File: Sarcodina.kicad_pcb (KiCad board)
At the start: 2 copper layers, 94 x 94 mm, 375 parts, among them SW1 SW_PUSH, SW10 SW_PUSH, SW11 SW_PUSH, SW12 SW_PUSH, SW13 SW_PUSH, SW14 SW_PUSH, SW15 SW_PUSH, SW16 SW_PUSH, SW17 SW_PUSH, SW18 SW_PUSH, SW19 SW_PUSH, SW2 SW_PUSH, SW20 SW_PUSH, SW21 SW_PUSH, SW22 SW_PUSH, SW23 SW_PUSH, SW24 SW_PUSH, SW25 SW_PUSH, SW3 SW_PUSH, SW4 SW_PUSH, SW5 SW_PUSH, SW6 SW_PUSH, SW7 SW_PUSH, SW8 SW_PUSH, SW9 SW_PUSH

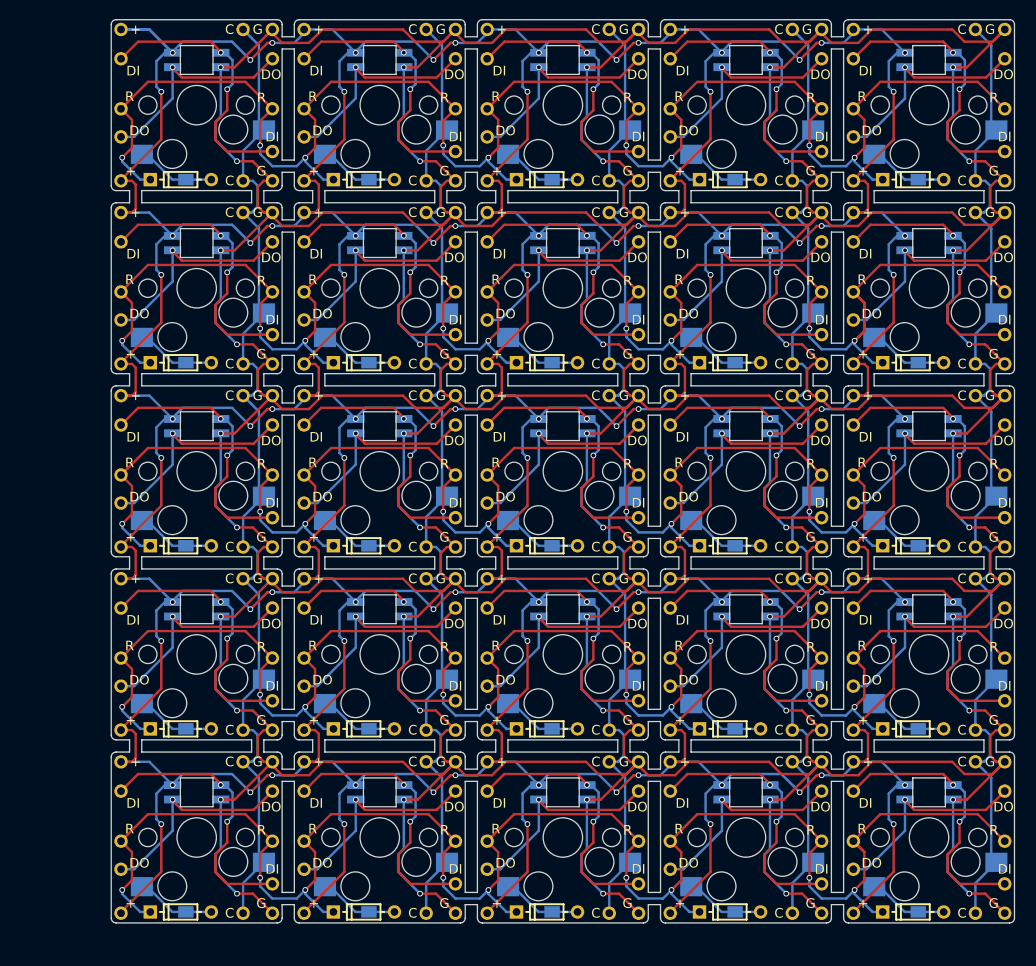
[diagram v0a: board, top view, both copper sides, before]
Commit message: Changed to a develop branch to update the pcb.
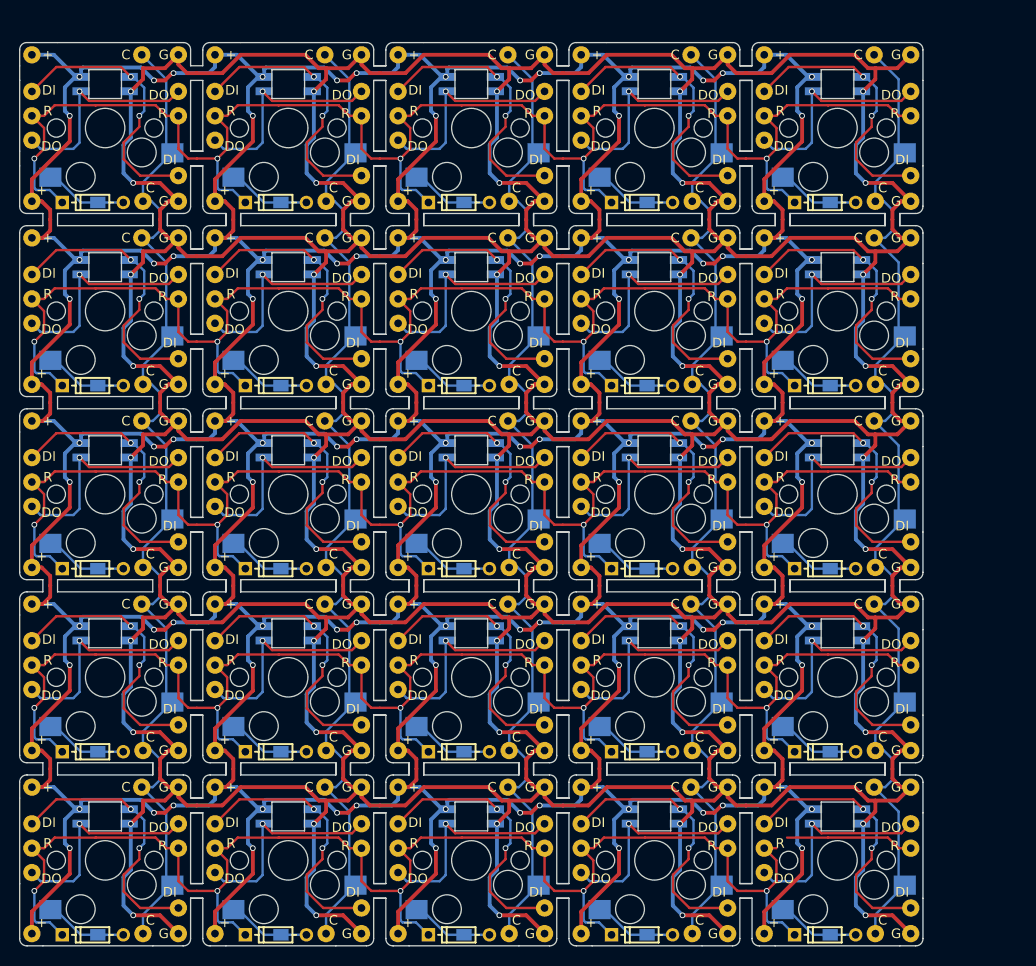
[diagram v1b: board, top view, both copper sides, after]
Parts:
- removed ** (x7), **1, **10, **100, **101, **102, **103, **104, **105, **106, **107, **108, **109, **11, **110, **111, **112, **113, **114, **115, **116, **117, **118, **119, **12, **120, **121, **122, **123, **124, **125, **126, **127, **128, **129, **13, **130, **131, **132, **133, **134, **135, **136, **137, **138, **139, **14, **140, **141, **142, **143, **144, **145, **146, **147, **148, **149, **15, **150, **151, **152, **153, **154, **155, **156, **157, **158, **159, **16, **160, **161, **162, **163, **164, **165, **166, **167, **168, **17, **18, **19, **2, **20, **21, **22, **23, **24, **25, **26, **27, **28, **29, **3, **30, **31, **32, **33, **34, **35, **36, **37, **38, **39, **4, **40, **41, **42, **43, **44, **45, **46, **47, **48, **49, **5, **50, **51, **52, **53, **54, **55, **56, **57, **58, **59, **6, **60, **61, **62, **63, **64, **65, **66, **67, **68, **69, **7, **70, **71, **72, **73, **74, **75, **76, **77, **78, **79, **8, **80, **81, **82, **83, **84, **85, **86, **87, **88, **89, **9, **90, **91, **92, **93, **94, **95, **96, **97, **98, **99: Val**, kbd:1pin_conn_no_silkscreen
- removed 1, 10, 11, 12, 13, 14, 15, 16, 17, 18, 19, 2, 20, 21, 22, 23, 24, 25, 26, 27, 28, 29, 3, 30, 31, 32, 33, 34, 35, 36, 37, 38, 39, 4, 40, 41, 42, 43, 44, 45, 46, 47, 48, 49, 5, 50, 51, 52, 53, 54, 55, 56, 57, 58, 59, 6, 60, 61, 62, 63, 64, 65, 66, 67, 68, 69, 7, 70, 71, 72, 73, 74, 75, 76, 77, 78, 79, 8, 80, 81, 82, 83, 84, 85, 86, 87, 88, 89, 9, 90, 91, 92, 93, 94, 95, 96: , 
- removed the ? at (109.7, 49.3)
- removed the ? at (109.7, 30.2)
- removed the ? at (71.6, 30.2)
- removed the ? at (71.6, 49.3)
- removed the ? at (109.7, 106.4)
- removed the ? at (128.8, 49.3)
- removed the ? at (71.6, 68.3)
- removed the ? at (109.7, 87.4)
- removed the ? at (128.8, 30.2)
- removed the ? at (90.7, 106.4)
- removed the ? at (90.7, 30.2)
- removed the ? at (52.6, 49.3)
- removed the ? at (71.6, 87.4)
- removed the ? at (128.8, 87.4)
- removed the ? at (52.6, 87.4)
- removed the ? at (52.6, 35.4)
- removed the ? at (52.6, 68.3)
- removed the ? at (90.7, 68.3)
- removed the ? at (68.3, 35.4)
- removed the ? at (109.7, 68.3)
- removed the ? at (128.8, 68.3)
- removed the ? at (90.7, 87.4)
- removed the ? at (128.8, 106.4)
- removed the ? at (52.6, 38.4)
- removed the ? at (90.7, 49.3)
- removed the ? at (65.3, 27.2)
- removed the ? at (52.6, 106.4)
- removed the ? at (52.6, 30.2)
- removed the ? at (71.6, 106.4)
- removed the D at (131.8, 119.0)
- removed the D at (55.6, 61.8)
- removed the D at (74.7, 119.0)
- removed the D at (93.7, 80.9)
- removed the D at (112.8, 42.8)
- removed the D at (74.7, 80.9)
- removed the D at (74.7, 99.9)
- removed the D at (93.7, 61.8)
- removed the D at (131.8, 42.8)
- removed the D at (112.8, 99.9)
- removed the D at (112.8, 61.8)
- removed the D at (93.7, 119.0)
- removed the D at (55.6, 80.9)
- removed the D at (55.6, 99.9)
- removed the D at (112.8, 119.0)
- removed the D at (93.7, 42.8)
- removed the D at (74.7, 61.8)
- removed the D at (131.8, 80.9)
- removed the D at (55.6, 119.0)
- removed the D at (74.7, 42.8)
- removed the D at (131.8, 61.8)
- removed the D at (112.8, 80.9)
- removed the D at (55.6, 42.8)
- removed the D at (93.7, 99.9)
- removed the D at (131.8, 99.9)
- removed the L1 at (79.5, 30.4)
- removed the L1 at (136.7, 68.5)
- removed the L1 at (79.5, 87.5)
- removed the L1 at (136.7, 49.4)
- removed the L1 at (79.5, 106.6)
- removed the L1 at (98.6, 87.5)
- removed the L1 at (79.5, 49.4)
- removed the L1 at (60.5, 87.5)
- removed the L1 at (79.5, 68.5)
- removed the L1 at (98.6, 49.4)
- removed the L1 at (136.7, 87.5)
- removed the L1 at (98.6, 106.6)
- removed the L1 at (117.6, 68.5)
- removed the L1 at (98.6, 68.5)
- removed the L1 at (136.7, 106.6)
- removed the L1 at (117.6, 106.6)
- removed the L1 at (136.7, 30.4)
- removed the L1 at (60.5, 30.4)
- removed the L1 at (60.5, 68.5)
- removed the L1 at (117.6, 49.4)
- removed the L1 at (117.6, 30.4)
- removed the L1 at (98.6, 30.4)
- removed the L1 at (60.5, 106.6)
- removed the L1 at (60.5, 49.4)
- removed the L1 at (117.6, 87.5)
- removed SW1, SW10, SW11, SW12, SW13, SW14, SW15, SW16, SW17, SW18, SW19, SW2, SW20, SW21, SW22, SW23, SW24, SW25, SW3, SW4, SW5, SW6, SW8, SW9: SW_PUSH, kbd:CherryMX_Hotswap_single_side
- removed the SW7 at (79.5, 54.1)
- added ?: , , F.Cu at (119.5, 74.3)
- added ?: , , F.Cu at (77.6, 90.8)
- added ?: , , F.Cu at (54.9, 83.2)
- added ?: , , F.Cu at (73.8, 106.0)
- added ?: , , F.Cu at (115.7, 112.4)
- added ?: , , F.Cu at (115.7, 102.2)
- added ?: , , F.Cu at (77.6, 64.1)
- added ?: , , F.Cu at (134.7, 42.4)
- added ?: , , F.Cu at (81.4, 106.0)
- added ?: , , F.Cu at (96.6, 36.2)
- added ?: , , F.Cu at (58.5, 83.2)
- added ?: , , F.Cu at (119.5, 71.7)
- added ?: , , F.Cu at (62.4, 121.3)
- added ?: , , F.Cu at (93.0, 83.2)
- added ?: , , F.Cu at (81.4, 52.7)
- added ?: , , F.Cu at (100.5, 36.2)
- added ?: , , F.Cu at (81.4, 95.9)
- added ?: , , F.Cu at (115.7, 29.8)
- added ?: , , F.Cu at (111.9, 48.9)
- added ?: , , F.Cu at (112.0, 45.1)
- added ?: , , F.Cu at (96.6, 42.4)
- added ?: , , F.Cu at (100.5, 90.8)
- added ?: , , F.Cu at (119.5, 83.2)
- added ?: , , F.Cu at (96.6, 80.5)
- added ?: , , F.Cu at (100.5, 71.7)
- added ?: , , F.Cu at (115.7, 36.2)
- added ?: , , F.Cu at (81.4, 48.9)
- added ?: , , F.Cu at (112.0, 83.2)
- added ?: , , F.Cu at (58.5, 109.8)
- added ?: , , F.Cu at (43.3, 87.0)
- added ?: , , F.Cu at (96.6, 33.6)
- added ?: , , F.Cu at (58.5, 71.7)
- added ?: , , F.Cu at (93.0, 121.3)
- added ?: , , F.Cu at (58.5, 64.1)
- added ?: , , F.Cu at (96.6, 106.0)
- added ?: , , F.Cu at (73.9, 83.2)
- added ?: , , F.Cu at (77.6, 109.8)
- added ?: , , F.Cu at (62.4, 55.2)
- added ?: , , F.Cu at (73.8, 29.8)
- added ?: , , F.Cu at (43.3, 57.8)
- added ?: , , F.Cu at (93.0, 45.1)
- added ?: , , F.Cu at (54.7, 48.9)
- added ?: , , F.Cu at (134.7, 55.2)
- added ?: , , F.Cu at (77.6, 55.2)
- added ?: , , F.Cu at (73.9, 121.3)
- added ?: , , F.Cu at (77.6, 80.5)
- added ?: , , F.Cu at (93.0, 64.1)
- added ?: , , F.Cu at (43.3, 121.3)
- added ?: , , F.Cu at (131.1, 64.1)
- added ?: , , F.Cu at (134.7, 109.8)
- added ?: , , F.Cu at (119.5, 45.1)
- added ?: , , F.Cu at (130.9, 29.8)
- added ?: , , F.Cu at (96.6, 29.8)
- added ?: , , F.Cu at (115.7, 87.0)
- added ?: , , F.Cu at (131.1, 83.2)
- added ?: , , F.Cu at (134.7, 99.5)
- added ?: , , F.Cu at (100.5, 95.9)
- added ?: , , F.Cu at (134.7, 36.2)
- added ?: , , F.Cu at (62.4, 106.0)
- added ?: , , F.Cu at (134.7, 93.3)
- added ?: , , F.Cu at (81.4, 83.2)
- added ?: , , F.Cu at (77.6, 99.5)
- added ?: , , F.Cu at (115.7, 109.8)
- added ?: , , F.Cu at (92.8, 106.0)
- added ?: , , F.Cu at (62.4, 36.2)
- added ?: , , F.Cu at (134.7, 33.6)
- added ?: , , F.Cu at (100.5, 83.2)
- added ?: , , F.Cu at (100.5, 67.9)
- added ?: , , F.Cu at (100.5, 114.9)
- added ?: , , F.Cu at (81.4, 76.8)
- added ?: , , F.Cu at (62.4, 57.8)
- added ?: , , F.Cu at (81.4, 38.7)
- added ?: , , F.Cu at (81.4, 29.8)
- added ?: , , F.Cu at (77.6, 33.6)
- added ?: , , F.Cu at (62.4, 71.7)
- added ?: , , F.Cu at (58.5, 106.0)
- added ?: , , F.Cu at (96.6, 74.3)
- added ?: , , F.Cu at (92.8, 87.0)
- added ?: , , F.Cu at (77.6, 112.4)
- added ?: , , F.Cu at (119.5, 67.9)
- added ?: , , F.Cu at (115.7, 45.1)
- added ?: , , F.Cu at (58.5, 29.8)
- added ?: , , F.Cu at (100.5, 64.1)
- added ?: , , F.Cu at (77.6, 36.2)
- added ?: , , F.Cu at (43.3, 106.0)
- added ?: , , F.Cu at (43.3, 76.8)
- added ?: , , F.Cu at (100.5, 45.1)
- added ?: , , F.Cu at (54.9, 64.1)
- added ?: , , F.Cu at (100.5, 102.2)
- added ?: , , F.Cu at (119.5, 36.2)
- added ?: , , F.Cu at (58.5, 102.2)
- added ?: , , F.Cu at (62.4, 29.8)
- added ?: , , F.Cu at (96.6, 83.2)
- added ?: , , F.Cu at (100.5, 121.3)
- added ?: , , F.Cu at (115.7, 93.3)
- added ?: , , F.Cu at (43.3, 45.1)
- added ?: , , F.Cu at (81.4, 57.8)
- added ?: , , F.Cu at (134.7, 102.2)
- added ?: , , F.Cu at (100.5, 57.8)
- added ?: , , F.Cu at (43.3, 36.2)
- added ?: , , F.Cu at (115.7, 99.5)
- added ?: , , F.Cu at (96.6, 67.9)
- added ?: , , F.Cu at (58.5, 87.0)
- added ?: , , F.Cu at (81.4, 67.9)
- added ?: , , F.Cu at (119.5, 87.0)
- added ?: , , F.Cu at (134.7, 71.7)
- added ?: , , F.Cu at (112.0, 102.2)
- added ?: , , F.Cu at (131.1, 121.3)
- added ?: , , F.Cu at (62.4, 114.9)
- added ?: , , F.Cu at (62.4, 76.8)
- added ?: , , F.Cu at (58.5, 74.3)
- added ?: , , F.Cu at (100.5, 76.8)
- added ?: , , F.Cu at (77.6, 52.7)
- added ?: , , F.Cu at (115.7, 61.4)
- added ?: , , F.Cu at (58.5, 36.2)
- added ?: , , F.Cu at (81.4, 90.8)
- added ?: , , F.Cu at (111.9, 106.0)
- added ?: , , F.Cu at (58.5, 80.5)
- added ?: , , F.Cu at (134.7, 118.6)
- added ?: , , F.Cu at (115.7, 48.9)
- added ?: , , F.Cu at (58.5, 52.7)
- added ?: , , F.Cu at (43.3, 38.7)
- added ?: , , F.Cu at (119.5, 52.7)
- added ?: , , F.Cu at (81.4, 102.2)
- added ?: , , F.Cu at (62.4, 45.1)
- added ?: , , F.Cu at (43.3, 55.2)
- added ?: , , F.Cu at (77.6, 29.8)
- added ?: , , F.Cu at (111.9, 87.0)
- added ?: , , F.Cu at (100.5, 87.0)
- added ?: , , F.Cu at (58.5, 99.5)
- added ?: , , F.Cu at (73.9, 45.1)
- added ?: , , F.Cu at (119.5, 57.8)
- added ?: , , F.Cu at (96.6, 52.7)
- added ?: , , F.Cu at (134.7, 83.2)
- added ?: , , F.Cu at (96.6, 99.5)
- added ?: , , F.Cu at (43.3, 33.6)
- added ?: , , F.Cu at (54.7, 67.9)
- added ?: , , F.Cu at (115.7, 33.6)
- added ?: , , F.Cu at (115.7, 74.3)
- added ?: , , F.Cu at (119.5, 33.6)
- added ?: , , F.Cu at (96.6, 45.1)
- added ?: , , F.Cu at (92.8, 48.9)
- added ?: , , F.Cu at (100.5, 93.3)
- added ?: , , F.Cu at (130.9, 106.0)
- added ?: , , F.Cu at (100.5, 112.4)
- added ?: , , F.Cu at (134.7, 87.0)
- added ?: , , F.Cu at (62.4, 83.2)
- added ?: , , F.Cu at (43.3, 83.2)
- added ?: , , F.Cu at (96.6, 121.3)
- added ?: , , F.Cu at (81.4, 112.4)
- added ?: , , F.Cu at (81.4, 114.9)
- added ?: , , F.Cu at (134.7, 121.3)
- added ?: , , F.Cu at (43.3, 52.7)
- added ?: , , F.Cu at (119.5, 114.9)
- added ?: , , F.Cu at (134.7, 29.8)
- added ?: , , F.Cu at (58.5, 118.6)
- added ?: , , F.Cu at (81.4, 45.1)
- added ?: , , F.Cu at (77.6, 74.3)
- added ?: , , F.Cu at (43.3, 67.9)
- added ?: , , F.Cu at (58.5, 45.1)
- added ?: , , F.Cu at (119.5, 112.4)
- added ?: , , F.Cu at (81.4, 55.2)
- added ?: , , F.Cu at (119.5, 90.8)
- added ?: , , F.Cu at (77.6, 48.9)
- added ?: , , F.Cu at (111.9, 29.8)
- added ?: , , F.Cu at (58.5, 121.3)
- added ?: , , F.Cu at (43.3, 74.3)
- added ?: , , F.Cu at (73.8, 48.9)
- added ?: , , F.Cu at (115.7, 118.6)
- added ?: , , F.Cu at (96.6, 61.4)
- added ?: , , F.Cu at (115.7, 42.4)
- added ?: , , F.Cu at (62.4, 38.7)
- added ?: , , F.Cu at (62.4, 90.8)
- added ?: , , F.Cu at (62.4, 52.7)
- added ?: , , F.Cu at (81.4, 74.3)
- added ?: , , F.Cu at (131.1, 102.2)
- added ?: , , F.Cu at (134.7, 67.9)
- added ?: , , F.Cu at (43.3, 64.1)
- added ?: , , F.Cu at (134.7, 112.4)
- added ?: , , F.Cu at (115.7, 64.1)
- added ?: , , F.Cu at (77.6, 42.4)
- added ?: , , F.Cu at (58.5, 93.3)
- added ?: , , F.Cu at (62.4, 102.2)
- added ?: , , F.Cu at (58.5, 33.6)
- added ?: , , F.Cu at (77.6, 118.6)
- added ?: , , F.Cu at (131.1, 45.1)
- added ?: , , F.Cu at (134.7, 74.3)
- added ?: , , F.Cu at (100.5, 55.2)
- added ?: , , F.Cu at (111.9, 67.9)
- added ?: , , F.Cu at (43.3, 114.9)
- added ?: , , F.Cu at (77.6, 83.2)
- added ?: , , F.Cu at (58.5, 112.4)
- added ?: , , F.Cu at (54.7, 106.0)
- added ?: , , F.Cu at (119.5, 76.8)
- added ?: , , F.Cu at (77.6, 102.2)
- added ?: , , F.Cu at (130.9, 67.9)
- added ?: , , F.Cu at (134.7, 48.9)
- added ?: , , F.Cu at (58.5, 67.9)
- added ?: , , F.Cu at (115.7, 55.2)
- added ?: , , F.Cu at (119.5, 102.2)
- added ?: , , F.Cu at (100.5, 29.8)
- added ?: , , F.Cu at (58.5, 48.9)
- added ?: , , F.Cu at (119.5, 38.7)
- added ?: , , F.Cu at (115.7, 83.2)
- added ?: , , F.Cu at (77.6, 71.7)
- added ?: , , F.Cu at (115.7, 67.9)
- added ?: , , F.Cu at (81.4, 109.8)
- added ?: , , F.Cu at (54.9, 102.2)
- added ?: , , F.Cu at (73.8, 87.0)
- added ?: , , F.Cu at (58.5, 61.4)
- added ?: , , F.Cu at (81.4, 121.3)
- added ?: , , F.Cu at (92.8, 29.8)
- added ?: , , F.Cu at (112.0, 121.3)
- added ?: , , F.Cu at (62.4, 112.4)
- added ?: , , F.Cu at (119.5, 55.2)
- added ?: , , F.Cu at (81.4, 64.1)
- added ?: , , F.Cu at (43.3, 112.4)
- added ?: , , F.Cu at (62.4, 64.1)
- added ?: , , F.Cu at (43.3, 29.8)
- added ?: , , F.Cu at (130.9, 87.0)
- added ?: , , F.Cu at (115.7, 71.7)
- added ?: , , F.Cu at (81.4, 93.3)
- added ?: , , F.Cu at (43.3, 102.2)
- added ?: , , F.Cu at (100.5, 38.7)
- added ?: , , F.Cu at (62.4, 67.9)
- added ?: , , F.Cu at (54.7, 29.8)
- added ?: , , F.Cu at (81.4, 33.6)
- added ?: , , F.Cu at (115.7, 106.0)
- added ?: , , F.Cu at (115.7, 52.7)
- added ?: , , F.Cu at (43.3, 71.7)
- added ?: , , F.Cu at (81.4, 36.2)
- added ?: , , F.Cu at (96.6, 87.0)
- added ?: , , F.Cu at (43.3, 93.3)
- added ?: , , F.Cu at (62.4, 87.0)
- added ?: , , F.Cu at (100.5, 33.6)
- added ?: , , F.Cu at (100.5, 48.9)
- added ?: , , F.Cu at (130.9, 48.9)
- added ?: , , F.Cu at (62.4, 33.6)
- added ?: , , F.Cu at (96.6, 112.4)
- added ?: , , F.Cu at (43.3, 109.8)
- added ?: , , F.Cu at (58.5, 55.2)
- added ?: , , F.Cu at (96.6, 109.8)
- added ?: , , F.Cu at (54.7, 87.0)
- added ?: , , F.Cu at (96.6, 90.8)
- added ?: , , F.Cu at (43.3, 90.8)
- added ?: , , F.Cu at (77.6, 45.1)
- added ?: , , F.Cu at (119.5, 121.3)
- added ?: , , F.Cu at (119.5, 64.1)
- added ?: , , F.Cu at (96.6, 118.6)
- added ?: , , F.Cu at (115.7, 90.8)
- added ?: , , F.Cu at (96.6, 71.7)
- added ?: , , F.Cu at (81.4, 87.0)
- added ?: , , F.Cu at (134.7, 61.4)
- added ?: , , F.Cu at (134.7, 90.8)
- added ?: , , F.Cu at (115.7, 80.5)
- added ?: , , F.Cu at (100.5, 52.7)
- added ?: , , F.Cu at (96.6, 55.2)
- added ?: , , F.Cu at (96.6, 48.9)
- added ?: , , F.Cu at (54.9, 121.3)
- added ?: , , F.Cu at (92.8, 67.9)
- added ?: , , F.Cu at (96.6, 102.2)
- added ?: , , F.Cu at (77.6, 87.0)
- added ?: , , F.Cu at (119.5, 93.3)
- added ?: , , F.Cu at (77.6, 67.9)
- added ?: , , F.Cu at (119.5, 29.8)
- added ?: , , F.Cu at (96.6, 64.1)
- added ?: , , F.Cu at (62.4, 74.3)
- added ?: , , F.Cu at (93.0, 102.2)
- added ?: , , F.Cu at (77.6, 93.3)
- added ?: , , F.Cu at (119.5, 95.9)
- added ?: , , F.Cu at (77.6, 106.0)
- added ?: , , F.Cu at (54.9, 45.1)
- added ?: , , F.Cu at (112.0, 64.1)
- added ?: , , F.Cu at (62.4, 109.8)
- added ?: , , F.Cu at (119.5, 48.9)
- added ?: , , F.Cu at (58.5, 90.8)
- added ?: , , F.Cu at (62.4, 95.9)
- added ?: , , F.Cu at (73.9, 102.2)
- added ?: , , F.Cu at (134.7, 106.0)
- added ?: , , F.Cu at (77.6, 121.3)
- added ?: , , F.Cu at (62.4, 93.3)
- added ?: , , F.Cu at (100.5, 106.0)
- added ?: , , F.Cu at (73.8, 67.9)
- added ?: , , F.Cu at (134.7, 45.1)
- added ?: , , F.Cu at (58.5, 42.4)
- added ?: , , F.Cu at (119.5, 106.0)
- added ?: , , F.Cu at (77.6, 61.4)
- added ?: , , F.Cu at (73.9, 64.1)
- added ?: , , F.Cu at (62.4, 48.9)
- added ?: , , F.Cu at (134.7, 80.5)
- added ?: , , F.Cu at (100.5, 109.8)
- added ?: , , F.Cu at (119.5, 109.8)
- added ?: , , F.Cu at (115.7, 121.3)
- added ?: , , F.Cu at (96.6, 93.3)
- added ?: , , F.Cu at (81.4, 71.7)
- added ?: , , F.Cu at (100.5, 74.3)
- added ?: , , F.Cu at (134.7, 64.1)
- added ?: , , F.Cu at (43.3, 95.9)
- added ?: , , F.Cu at (43.3, 48.9)
- added ?: , , F.Cu at (134.7, 52.7)
- added D: D, kbd:D3_hybrid_common_hole, F.Cu at (103.6, 64.2)
- added D: D, kbd:D3_hybrid_common_hole, F.Cu at (65.5, 83.3)
- added D: D, kbd:D3_hybrid_common_hole, F.Cu at (122.7, 64.2)
- added D: D, kbd:D3_hybrid_common_hole, F.Cu at (103.6, 121.4)
- added D: D, kbd:D3_hybrid_common_hole, F.Cu at (46.5, 64.2)
- added D: D, kbd:D3_hybrid_common_hole, F.Cu at (122.7, 121.4)
- added D: D, kbd:D3_hybrid_common_hole, F.Cu at (46.5, 83.3)
- added D: D, kbd:D3_hybrid_common_hole, F.Cu at (84.6, 64.2)
- added D: D, kbd:D3_hybrid_common_hole, F.Cu at (122.7, 83.3)
- added D: D, kbd:D3_hybrid_common_hole, F.Cu at (103.6, 45.2)
- added D: D, kbd:D3_hybrid_common_hole, F.Cu at (84.6, 83.3)
- added D: D, kbd:D3_hybrid_common_hole, F.Cu at (46.5, 121.4)
- added D: D, kbd:D3_hybrid_common_hole, F.Cu at (65.5, 102.3)
- added D: D, kbd:D3_hybrid_common_hole, F.Cu at (46.5, 45.2)
- added D: D, kbd:D3_hybrid_common_hole, F.Cu at (65.5, 45.2)
- added D: D, kbd:D3_hybrid_common_hole, F.Cu at (84.6, 102.3)
- added D: D, kbd:D3_hybrid_common_hole, F.Cu at (65.5, 64.2)
- added D: D, kbd:D3_hybrid_common_hole, F.Cu at (122.7, 102.3)
- added D: D, kbd:D3_hybrid_common_hole, F.Cu at (84.6, 121.4)
- added D: D, kbd:D3_hybrid_common_hole, F.Cu at (103.6, 102.3)
- added D: D, kbd:D3_hybrid_common_hole, F.Cu at (122.7, 45.2)
- added D: D, kbd:D3_hybrid_common_hole, F.Cu at (84.6, 45.2)
- added D: D, kbd:D3_hybrid_common_hole, F.Cu at (103.6, 83.3)
- added D: D, kbd:D3_hybrid_common_hole, F.Cu at (46.5, 102.3)
- added D: D, kbd:D3_hybrid_common_hole, F.Cu at (65.5, 121.4)
- added L1: SK6812MINI, kbd:YS-SK6812MINI-E, B.Cu at (70.0, 51.9)
- added L1: SK6812MINI, kbd:YS-SK6812MINI-E, B.Cu at (127.1, 32.9)
- added L1: SK6812MINI, kbd:YS-SK6812MINI-E, B.Cu at (108.1, 90.0)
- added L1: SK6812MINI, kbd:YS-SK6812MINI-E, B.Cu at (70.0, 109.1)
- added L1: SK6812MINI, kbd:YS-SK6812MINI-E, B.Cu at (108.1, 32.9)
- added L1: SK6812MINI, kbd:YS-SK6812MINI-E, B.Cu at (108.1, 51.9)
- added L1: SK6812MINI, kbd:YS-SK6812MINI-E, B.Cu at (50.9, 51.9)
- added L1: SK6812MINI, kbd:YS-SK6812MINI-E, B.Cu at (50.9, 109.1)
- added L1: SK6812MINI, kbd:YS-SK6812MINI-E, B.Cu at (89.0, 51.9)
- added L1: SK6812MINI, kbd:YS-SK6812MINI-E, B.Cu at (70.0, 71.0)
- added L1: SK6812MINI, kbd:YS-SK6812MINI-E, B.Cu at (127.1, 109.1)
- added L1: SK6812MINI, kbd:YS-SK6812MINI-E, B.Cu at (89.0, 109.1)
- added L1: SK6812MINI, kbd:YS-SK6812MINI-E, B.Cu at (50.9, 90.0)
- added L1: SK6812MINI, kbd:YS-SK6812MINI-E, B.Cu at (89.0, 32.9)
- added L1: SK6812MINI, kbd:YS-SK6812MINI-E, B.Cu at (127.1, 71.0)
- added L1: SK6812MINI, kbd:YS-SK6812MINI-E, B.Cu at (50.9, 32.9)
- added L1: SK6812MINI, kbd:YS-SK6812MINI-E, B.Cu at (89.0, 90.0)
- added L1: SK6812MINI, kbd:YS-SK6812MINI-E, B.Cu at (127.1, 51.9)
- added L1: SK6812MINI, kbd:YS-SK6812MINI-E, B.Cu at (108.1, 71.0)
- added L1: SK6812MINI, kbd:YS-SK6812MINI-E, B.Cu at (50.9, 71.0)
- added L1: SK6812MINI, kbd:YS-SK6812MINI-E, B.Cu at (127.1, 90.0)
- added L1: SK6812MINI, kbd:YS-SK6812MINI-E, B.Cu at (70.0, 90.0)
- added L1: SK6812MINI, kbd:YS-SK6812MINI-E, B.Cu at (108.1, 109.1)
- added L1: SK6812MINI, kbd:YS-SK6812MINI-E, B.Cu at (89.0, 71.0)
- added L1: SK6812MINI, kbd:YS-SK6812MINI-E, B.Cu at (70.0, 32.9)
- added SW7: SW_PUSH, kbd:CherryMX_Hotswap_single_side, F.Cu at (70.0, 113.6)
- added SW7: SW_PUSH, kbd:CherryMX_Hotswap_single_side, F.Cu at (50.9, 56.5)
- added SW7: SW_PUSH, kbd:CherryMX_Hotswap_single_side, F.Cu at (70.0, 75.5)
- added SW7: SW_PUSH, kbd:CherryMX_Hotswap_single_side, F.Cu at (127.1, 113.6)
- added SW7: SW_PUSH, kbd:CherryMX_Hotswap_single_side, F.Cu at (89.0, 37.4)
- added SW7: SW_PUSH, kbd:CherryMX_Hotswap_single_side, F.Cu at (127.1, 56.5)
- added SW7: SW_PUSH, kbd:CherryMX_Hotswap_single_side, F.Cu at (127.1, 75.5)
- added SW7: SW_PUSH, kbd:CherryMX_Hotswap_single_side, F.Cu at (108.1, 37.4)
- added SW7: SW_PUSH, kbd:CherryMX_Hotswap_single_side, F.Cu at (50.9, 94.6)
- added SW7: SW_PUSH, kbd:CherryMX_Hotswap_single_side, F.Cu at (89.0, 75.5)
- added SW7: SW_PUSH, kbd:CherryMX_Hotswap_single_side, F.Cu at (108.1, 94.6)
- added SW7: SW_PUSH, kbd:CherryMX_Hotswap_single_side, F.Cu at (70.0, 56.5)
- added SW7: SW_PUSH, kbd:CherryMX_Hotswap_single_side, F.Cu at (108.1, 56.5)
- added SW7: SW_PUSH, kbd:CherryMX_Hotswap_single_side, F.Cu at (50.9, 37.4)
- added SW7: SW_PUSH, kbd:CherryMX_Hotswap_single_side, F.Cu at (50.9, 75.5)
- added SW7: SW_PUSH, kbd:CherryMX_Hotswap_single_side, F.Cu at (89.0, 113.6)
- added SW7: SW_PUSH, kbd:CherryMX_Hotswap_single_side, F.Cu at (127.1, 37.4)
- added SW7: SW_PUSH, kbd:CherryMX_Hotswap_single_side, F.Cu at (89.0, 56.5)
- added SW7: SW_PUSH, kbd:CherryMX_Hotswap_single_side, F.Cu at (89.0, 94.6)
- added SW7: SW_PUSH, kbd:CherryMX_Hotswap_single_side, F.Cu at (108.1, 75.5)
- added SW7: SW_PUSH, kbd:CherryMX_Hotswap_single_side, F.Cu at (70.0, 94.6)
- added SW7: SW_PUSH, kbd:CherryMX_Hotswap_single_side, F.Cu at (108.1, 113.6)
- added SW7: SW_PUSH, kbd:CherryMX_Hotswap_single_side, F.Cu at (70.0, 37.4)
- added SW7: SW_PUSH, kbd:CherryMX_Hotswap_single_side, F.Cu at (50.9, 113.6)
- added SW7: SW_PUSH, kbd:CherryMX_Hotswap_single_side, F.Cu at (127.1, 94.6)
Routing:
- net GND: track 1096.4 -> 1067.6 mm
- net Net-(D1-Pad2): track 194.6 -> 216.9 mm
- net VCC: track 1001.6 -> 1021.2 mm
- net row1: track 190.0 -> 172.4 mm, vias 9 -> 5
- net row4: track 185.7 -> 170.8 mm, vias 9 -> 5
- net row3: track 184.0 -> 172.4 mm, vias 9 -> 5
- net row0: track 184.0 -> 172.4 mm, vias 9 -> 5
- net row2: track 184.0 -> 172.4 mm, vias 9 -> 5
- net unconnected-(L1-Pad4): track 703.0 -> 708.6 mm
- net col4: track 110.5 -> 115.3 mm
- net col3: track 110.5 -> 115.3 mm
- net col1: track 110.5 -> 115.3 mm
- net col2: track 110.5 -> 115.3 mm
- net unconnected-(L1-Pad2): track 546.1 -> 550.8 mm
- net col0: track 111.3 -> 115.3 mm
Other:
- outline, holes or cut-outs redrawn
